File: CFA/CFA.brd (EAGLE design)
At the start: 60.9 x 83.5 mm, 77 parts, among them IC1 OPA345P, Q1 BC550C, Q10 BC560C, Q11 BC550C, Q12 MJE15030, Q13 MJE15031, Q14 MJE15030, Q15 BC560C, Q16 MJE15031, Q17 MJE15031, Q18 BC560C, Q19 BC550C, Q2 BC550C, Q20 BC550C, Q21 MJE15030, Q22 BC560C, Q23 BC560C, Q24 BC550C, Q25 BC550C, Q27 PZTA56, Q28 PZTA06SOT-223, Q3 BC560C, Q4 BC560C, Q5 MJE15030, Q6 BC560C, Q7 BC550C, Q8 BC550C, Q9 BC560C, X1 MKDSN1,5/2-5,08, X2 MKDSN1,5/2-5,08

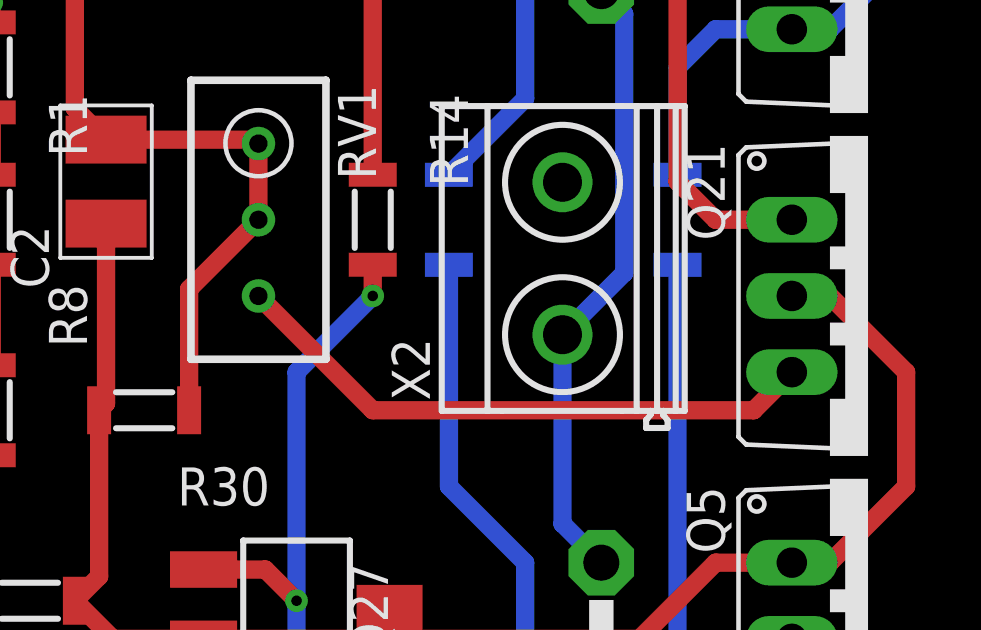
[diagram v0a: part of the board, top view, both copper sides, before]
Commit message: VCFA2
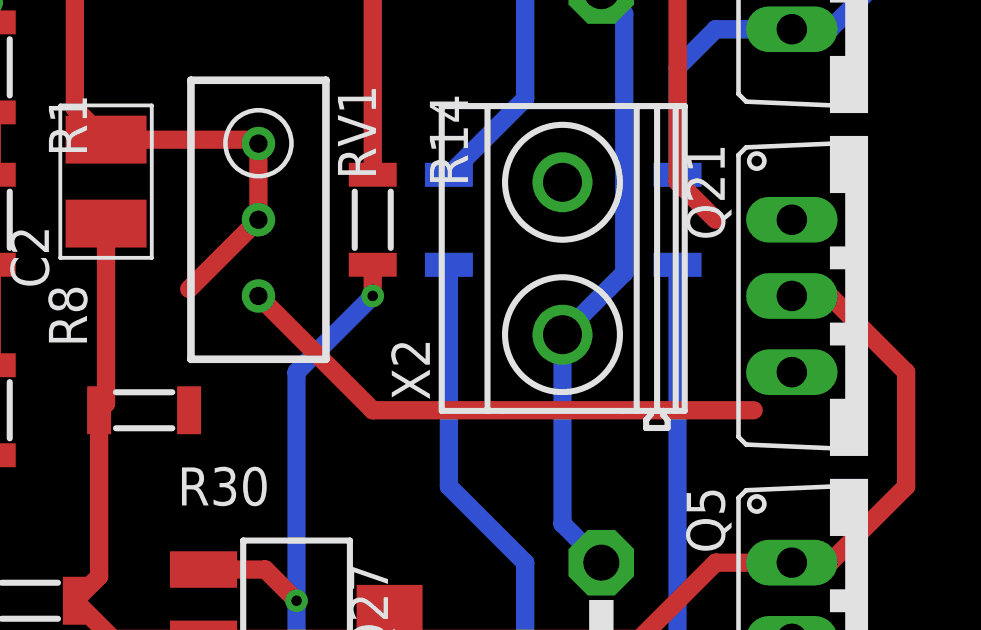
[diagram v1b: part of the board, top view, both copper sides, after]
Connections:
- net N$1: now also Q21.B, R30.1; no longer Q21.E
- net N$48: now also Q21.E; no longer Q21.B, R30.1
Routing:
- net N$48: track 84.3 -> 77.8 mm
- net N$1: track 19.9 -> 18.1 mm
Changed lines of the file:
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@@
 <?xml version="1.0" encoding="utf-8"?>
 <!DOCTYPE eagle SYSTEM "eagle.dtd">
-<eagle version="9.3.1">
+<eagle version="9.4.2">
 <drawing>
 <settings>
-<setting alwaysvectorfont="yes"/>
+<setting alwaysvectorfont="no"/>
 <setting verticaltext="up"/>
 </settings>
@@
 </signal>
 <signal name="N$48">
-<contactref element="Q21" pad="B"/>
-<contactref element="R30" pad="1"/>
 <contactref element="R15" pad="2"/>
 <contactref element="Q28" pad="2"/>
@@
 <wire x1="41.199" y1="55.88" x2="50.8" y2="55.88" width="0.6096" layer="1"/>
 <wire x1="50.8" y1="55.88" x2="54.61" y2="55.88" width="0.6096" layer="1"/>
-<wire x1="54.61" y1="44.45" x2="52.07" y2="44.45" width="0.6096" layer="1"/>
 <wire x1="52.07" y1="44.45" x2="50.8" y2="45.72" width="0.6096" layer="1"/>
 <wire x1="50.8" y1="45.72" x2="50.8" y2="55.88" width="0.6096" layer="1"/>
@@
 <wire x1="36.7" y1="47.12" x2="31.75" y2="47.12" width="0.6096" layer="1"/>
 <wire x1="36.83" y1="44.45" x2="36.83" y2="46.99" width="0.6096" layer="1"/>
-<wire x1="34.52" y1="38.1" x2="34.52" y2="42.14" width="0.6096" layer="1"/>
 <wire x1="34.52" y1="42.14" x2="36.83" y2="44.45" width="0.6096" layer="1"/>
+<contactref element="Q21" pad="E"/>
+<wire x1="52.07" y1="44.45" x2="54.61" y2="39.37" width="0" layer="19" extent="1-1"/>
 </signal>
 <signal name="N$35">
@@
 <signal name="N$1">
 <contactref element="RV1" pad="3"/>
-<contactref element="Q21" pad="E"/>
 <wire x1="36.83" y1="41.91" x2="40.64" y2="38.1" width="0.6096" layer="1"/>
 <wire x1="40.64" y1="38.1" x2="53.34" y2="38.1" width="0.6096" layer="1"/>
-<wire x1="53.34" y1="38.1" x2="54.61" y2="39.37" width="0.6096" layer="1"/>
+<contactref element="Q21" pad="B"/>
+<contactref element="R30" pad="1"/>
+<wire x1="53.34" y1="38.1" x2="54.61" y2="44.45" width="0" layer="19" extent="1-1"/>
+<wire x1="34.52" y1="38.1" x2="36.83" y2="41.91" width="0" layer="19" extent="1-1"/>
 </signal>
 <signal name="N$17">
